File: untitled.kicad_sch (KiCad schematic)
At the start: 10 parts, among them Q1 NMOS, Q10 NMOS, Q2 NMOS, Q3 NMOS, Q4 NMOS, Q5 NMOS, Q6 NMOS, Q7 NMOS, Q8 NMOS, Q9 NMOS

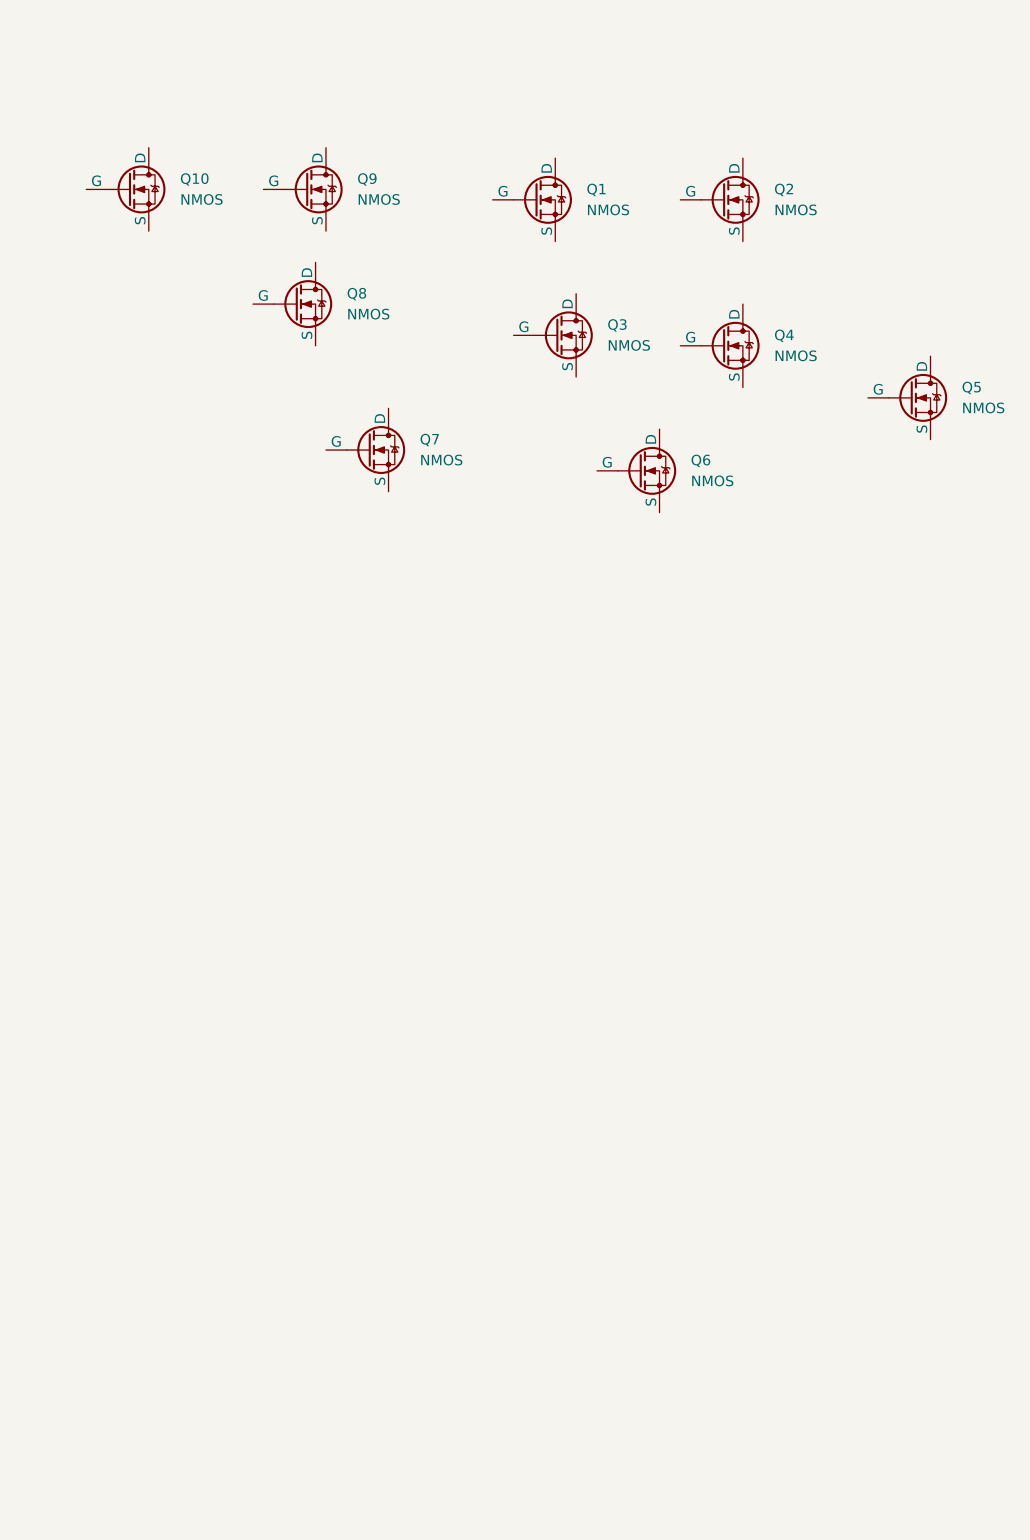
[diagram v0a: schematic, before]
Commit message: Much more progress
hi mom
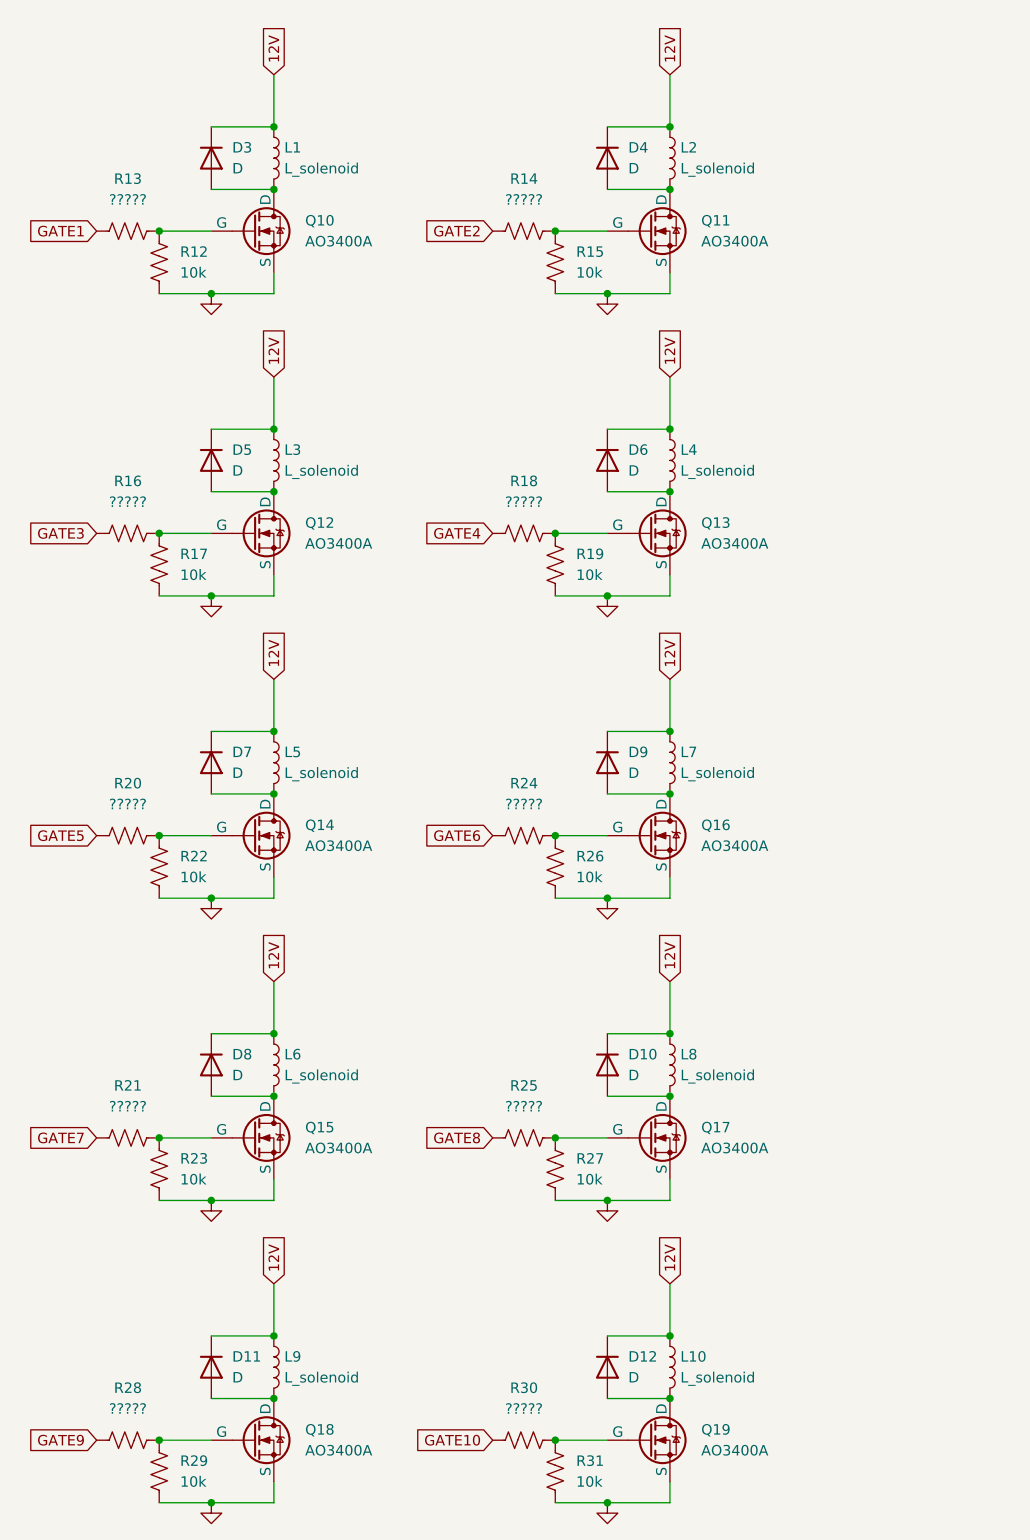
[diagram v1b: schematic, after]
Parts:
- removed Q1, Q2, Q3, Q4, Q5, Q6, Q7, Q8, Q9: NMOS, symbol Simulation_SPICE:NMOS
- added D10, D11, D12, D3, D4, D5, D6, D7, D8, D9: D, symbol Device:D
- added L1, L10, L2, L3, L4, L5, L6, L7, L8, L9: L_solenoid, symbol Device:L
- added Q11, Q12, Q13, Q14, Q15, Q16, Q17, Q18, Q19: AO3400A, symbol Simulation_SPICE:NMOS
- added R12, R15, R17, R19, R22, R23, R26, R27, R29, R31: 10k, symbol Device:R_US
- added R13, R14, R16, R18, R20, R21, R24, R25, R28, R30: ?????, symbol Device:R_US
- Q10: value NMOS -> AO3400A
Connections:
- net at Q10.1 (D): now also D3.2 (A), L1.2
- net at Q10.2 (G): now also R12.1, R13.2
- net GND: now reaches Q10.3 (S)
- net GND: now also Q11.3 (S), Q12.3 (S), Q13.3 (S), Q14.3 (S), Q15.3 (S), Q16.3 (S), Q17.3 (S), Q18.3 (S), Q19.3 (S), R12.2, R15.2, R17.2, R19.2, R22.2, R23.2, R26.2, R27.2, R29.2, R31.2
- new net: D9.2 (A), L7.2, Q16.1 (D)
- new net: D11.2 (A), L9.2, Q18.1 (D)
- new net: D12.2 (A), L10.2, Q19.1 (D)
- new net: Q15.2 (G), R21.2, R23.1
- new net: Q18.2 (G), R28.2, R29.1
- new net: D8.2 (A), L6.2, Q15.1 (D)
- new net: Q16.2 (G), R24.2, R26.1
- new net: D4.2 (A), L2.2, Q11.1 (D)
- new net: Q11.2 (G), R14.2, R15.1
- new net: Q19.2 (G), R30.2, R31.1
- new net: D5.2 (A), L3.2, Q12.1 (D)
- new net: Q12.2 (G), R16.2, R17.1
- new net: D6.2 (A), L4.2, Q13.1 (D)
- new net: D10.2 (A), L8.2, Q17.1 (D)
- new net: Q17.2 (G), R25.2, R27.1
- new net: D7.2 (A), L5.2, Q14.1 (D)
- new net: Q14.2 (G), R20.2, R22.1
- new net: Q13.2 (G), R18.2, R19.1
- new net 12V: D10.1 (K), D11.1 (K), D12.1 (K), D3.1 (K), D4.1 (K), D5.1 (K), D6.1 (K), D7.1 (K), D8.1 (K), D9.1 (K), L1.1, L10.1, L2.1, L3.1, L4.1, L5.1, L6.1, L7.1, L8.1, L9.1
- new net GATE1: R13.1
- new net GATE10: R30.1
- new net GATE2: R14.1
- new net GATE3: R16.1
- new net GATE4: R18.1
- new net GATE5: R20.1
- new net GATE6: R24.1
- new net GATE7: R21.1
- new net GATE8: R25.1
- new net GATE9: R28.1
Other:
- moved on the sheet: Q10
